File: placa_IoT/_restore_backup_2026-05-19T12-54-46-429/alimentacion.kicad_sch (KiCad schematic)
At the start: 8 parts, among them U1 RT9080-33GJ5, U2 RT9080-33GJ5

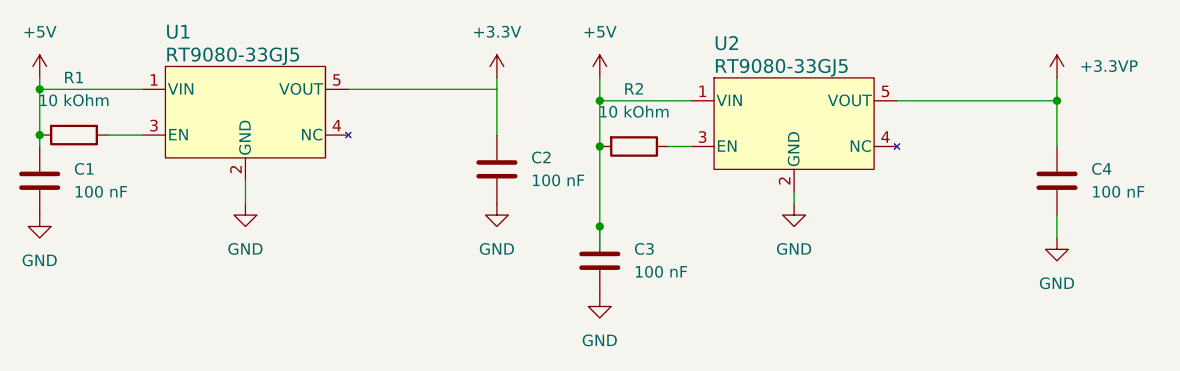
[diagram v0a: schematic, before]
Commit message: Alimentacion add
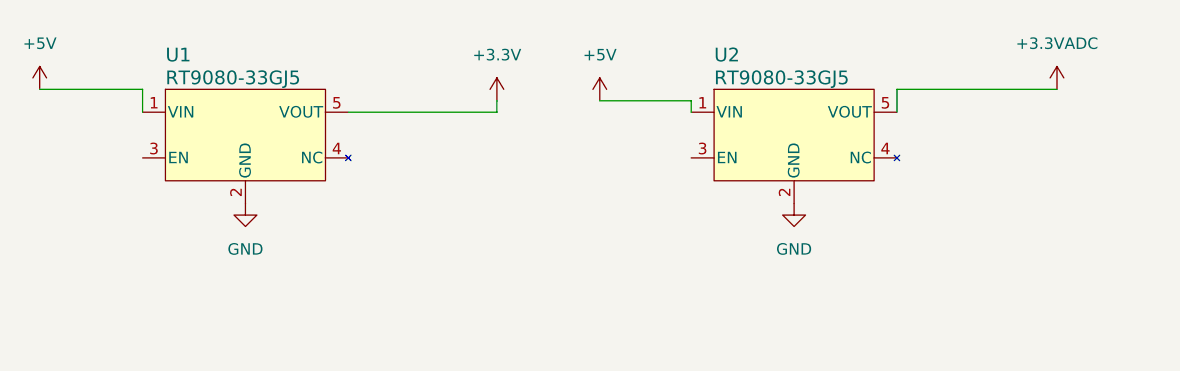
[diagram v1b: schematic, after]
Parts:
- removed C1, C2, C3, C4: 100 nF, Capacitor_SMD:C_0402_1005Metric, symbol Device:C
- removed R1, R2: 10 kOhm, Resistor_SMD:R_0402_1005Metric, symbol Device:R
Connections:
- net +3.3V: now also U1.5 (VOUT)
- net +3.3VP renamed +3.3VADC
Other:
- moved on the sheet: U1, U2
